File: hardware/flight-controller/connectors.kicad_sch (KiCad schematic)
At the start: 40 parts, among them J10 IDC-10, J3 IDC-10, J4 Conn_01x03, J5 Conn_01x03, J6 Conn_01x03, J7 IDC-10, J8 XT-60, J9 Conn_01x03

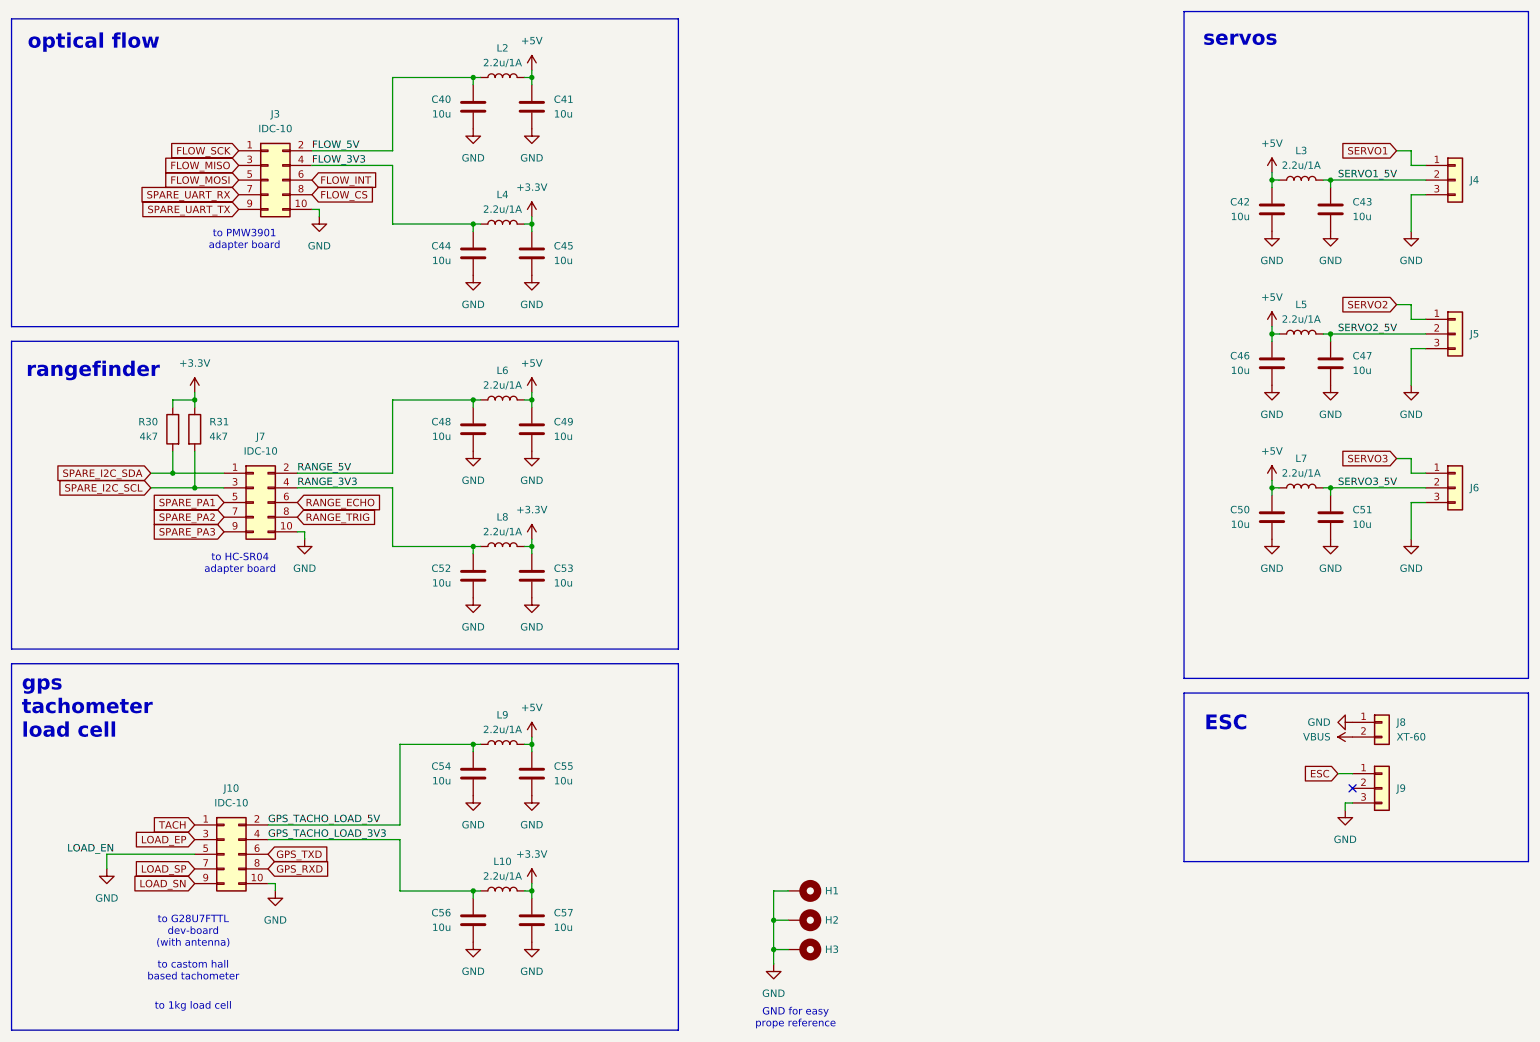
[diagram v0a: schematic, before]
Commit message: Mouser
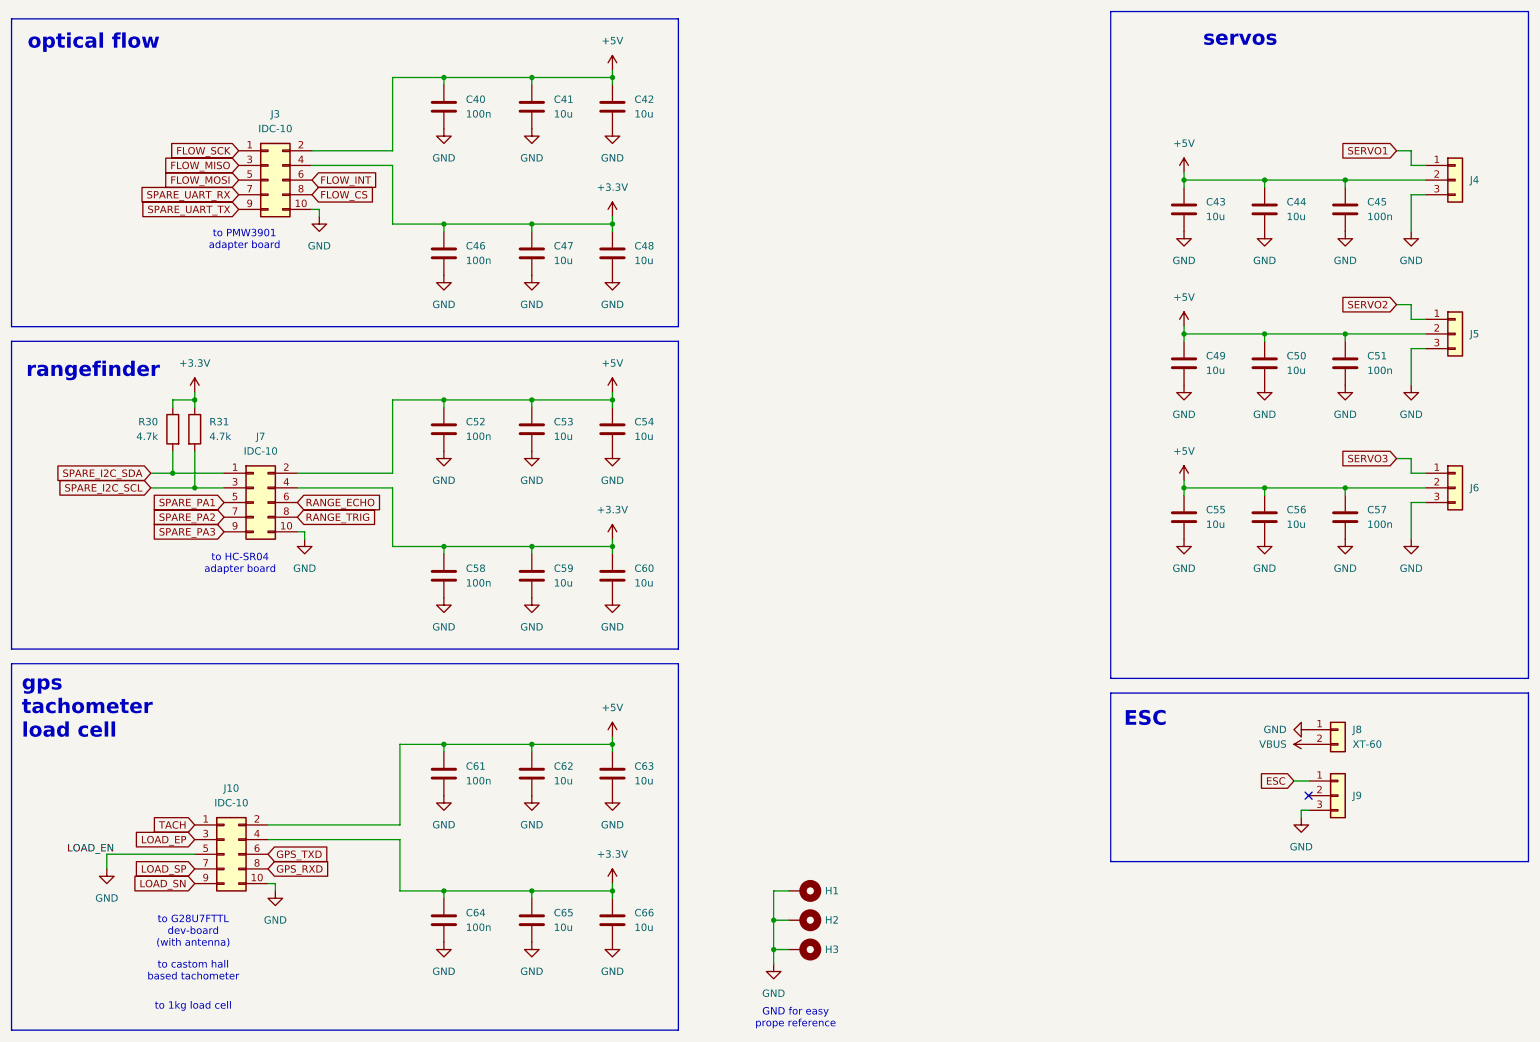
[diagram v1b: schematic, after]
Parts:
- removed L10, L2, L3, L4, L5, L6, L7, L8, L9: 2.2u/1A, Inductor_SMD:L_0603_1608Metric, symbol Device:L
- added C40, C45, C46, C51, C52, C57, C58, C61, C64: 100n, Capacitor_SMD:C_0603_1608Metric, symbol Device:C
- R30, R31: value 4k7 -> 4.7k
- renumbered C40 to C42, C42 to C43, C43 to C44, C44 to C47, C45 to C48, C46 to C49, C47 to C50, C48 to C53, C49 to C54, C50 to C55, C51 to C56, C52 to C59, C53 to C60, C54 to C62, C55 to C63, C56 to C65, C57 to C66
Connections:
- net FLOW_3V3 is gone; now on net +3.3V: C47.1, J3.4 (Pin_4)
- net FLOW_5V is gone; now on net +5V: C42.1, J3.2 (Pin_2)
- net GPS_TACHO_LOAD_3V3 is gone; now on net +3.3V: C65.1, J10.4 (Pin_4)
- net GPS_TACHO_LOAD_5V is gone; now on net +5V: C62.1, J10.2 (Pin_2)
- net RANGE_3V3 is gone; now on net +3.3V: C59.1, J7.4 (Pin_4)
- net RANGE_5V is gone; now on net +5V: C53.1, J7.2 (Pin_2)
- net SERVO1_5V is gone; now on net +5V: C44.1, J4.2 (Pin_2)
- net SERVO2_5V is gone; now on net +5V: C50.1, J5.2 (Pin_2)
- net SERVO3_5V is gone; now on net +5V: C56.1, J6.2 (Pin_2)
- net +3.3V: now also C46.1, C58.1, C64.1
- net +5V: now also C40.1, C45.1, C51.1, C52.1, C57.1, C61.1
- net GND: now also C40.2, C45.2, C46.2, C51.2, C52.2, C57.2, C58.2, C61.2, C64.2
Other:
- moved on the sheet: C42, C43, C44, C47, C48, C49, C50, C53, C54, C55, C56, C59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

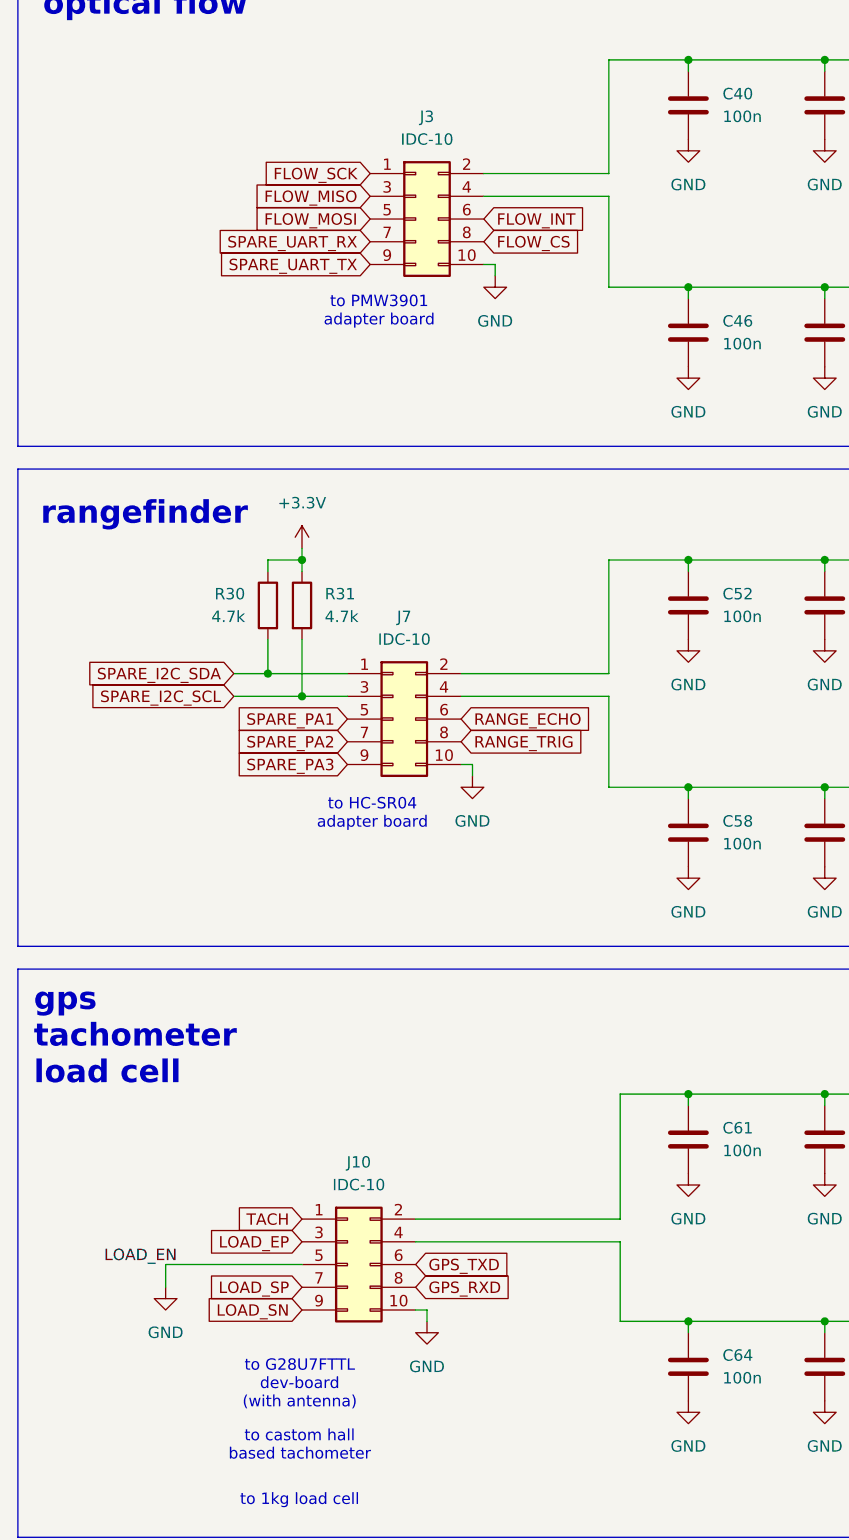
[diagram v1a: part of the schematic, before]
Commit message: routing: all signals routed
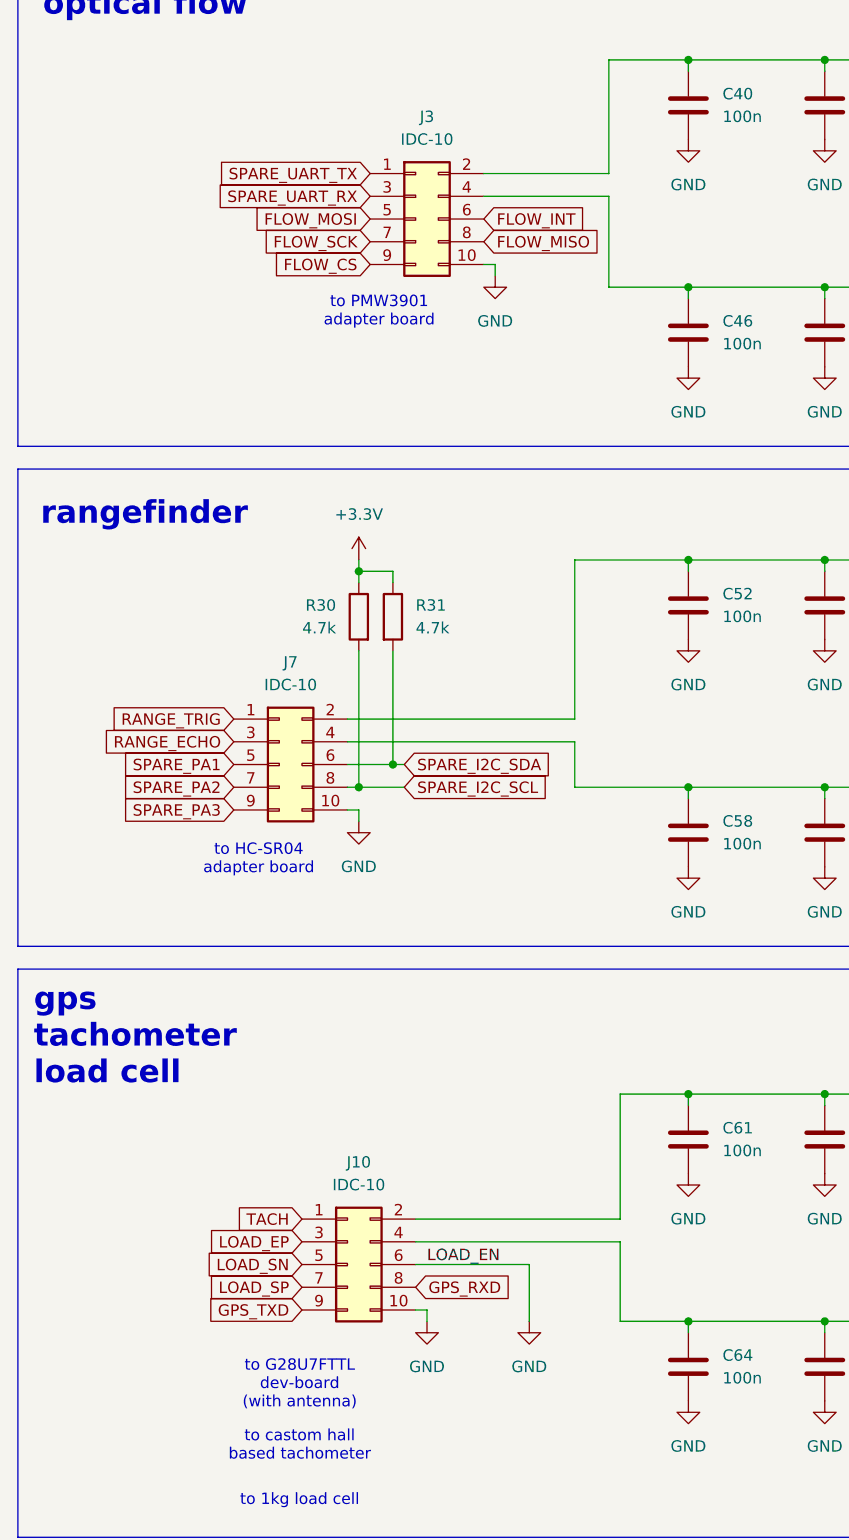
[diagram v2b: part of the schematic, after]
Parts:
- renumbered R31 to R30, R30 to R31
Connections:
- net FLOW_CS: now also J3.9 (Pin_9); no longer J3.8 (Pin_8)
- net FLOW_MISO: now also J3.8 (Pin_8); no longer J3.3 (Pin_3)
- net FLOW_SCK: now also J3.7 (Pin_7); no longer J3.1 (Pin_1)
- net GND: now also J10.6 (Pin_6); no longer J10.5 (Pin_5)
- net GPS_TXD: now also J10.9 (Pin_9); no longer J10.6 (Pin_6)
- net LOAD_SN: now also J10.5 (Pin_5); no longer J10.9 (Pin_9)
- net RANGE_ECHO: now also J7.3 (Pin_3); no longer J7.6 (Pin_6)
- net RANGE_TRIG: now also J7.1 (Pin_1); no longer J7.8 (Pin_8)
- net SPARE_I2C_SCL: now also J7.8 (Pin_8); no longer J7.3 (Pin_3)
- net SPARE_I2C_SDA: now also J7.6 (Pin_6); no longer J7.1 (Pin_1)
- net SPARE_UART_RX: now also J3.3 (Pin_3); no longer J3.7 (Pin_7)
- net SPARE_UART_TX: now also J3.1 (Pin_1); no longer J3.9 (Pin_9)
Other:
- moved on the sheet: J7, R30, R31
